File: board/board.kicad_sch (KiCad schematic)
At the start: 4 parts, among them J1 Conn_01x02_Pin, J2 Conn_01x02_Pin, J3 003_power

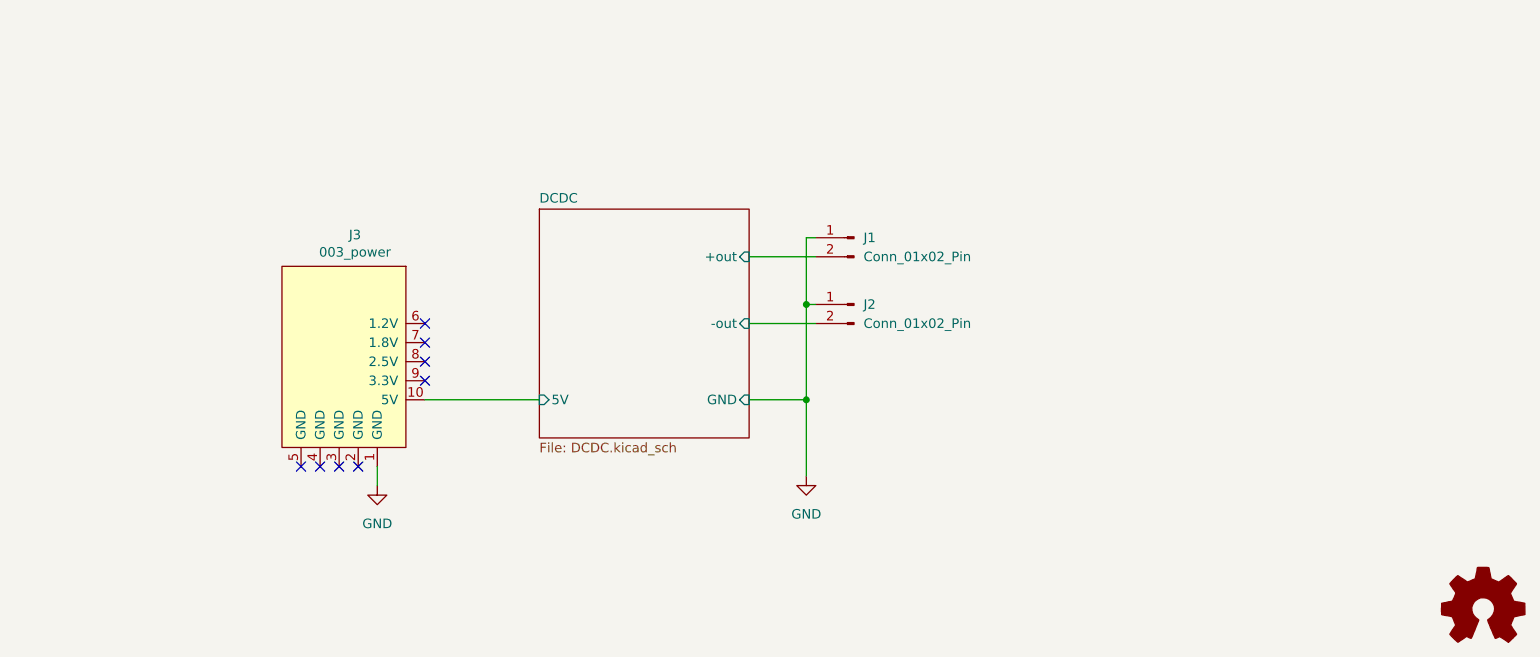
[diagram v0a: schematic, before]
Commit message: initial b148
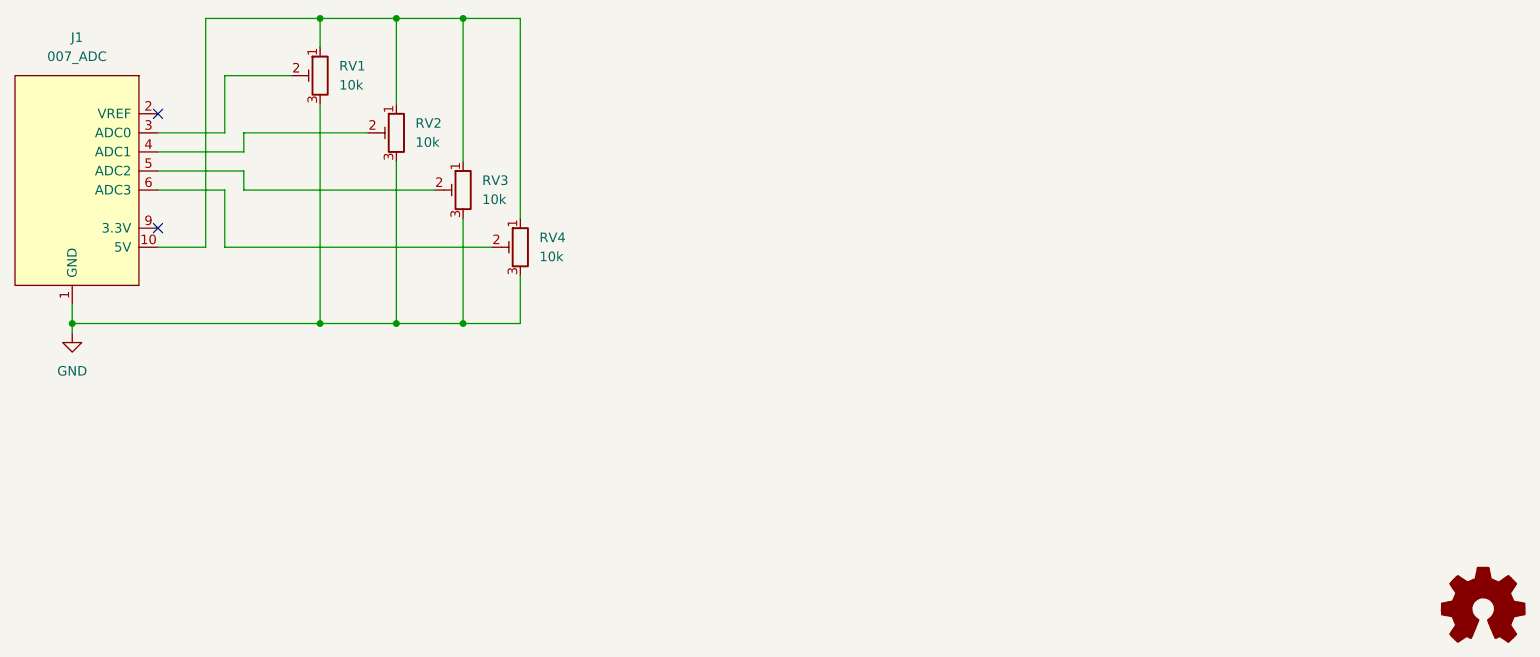
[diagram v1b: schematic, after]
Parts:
- removed J1, J2: Conn_01x02_Pin, Connector_PinHeader_2.54mm:PinHeader_1x02_P2.54mm_Vertical, symbol Connector:Conn_01x02_Pin
- removed J3: 003_power, on_edge:on_edge_2x05_device, symbol put_on_edge:003_power
- added J1: 007_ADC, on_edge:on_edge_2x05_device, symbol put_on_edge:007_ADC
- added RV1, RV2, RV3, RV4: 10k, Potentiometer_SMD:Potentiometer_Bourns_TC33X_Vertical, symbol Device:R_Potentiometer_Trim
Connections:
- net GND: now also J1.1 (GND), RV1.3, RV2.3, RV3.3, RV4.3
- new net: J1.10 (5V), RV1.1, RV2.1, RV3.1, RV4.1
- new net: J1.6 (ADC3), RV4.2
- new net: J1.3 (ADC0), RV1.2
- new net: J1.4 (ADC1), RV2.2
- new net: J1.5 (ADC2), RV3.2
- no-connect marks 8 -> 2
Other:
- removed sheet DCDC
